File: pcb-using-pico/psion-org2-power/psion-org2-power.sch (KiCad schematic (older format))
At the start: 47 parts, among them J1 Conn_02x08_Odd_Even, J2 Conn_02x08_Odd_Even, J3 Conn_01x27_Female, J4 Conn_02x08_Odd_Even, J5 Conn_01x11_Female, J6 Conn_01x02_Female, M1 P-CHANNEL-MOSFET, M2 P-CHANNEL-MOSFET, M3 AO3401, U1 ESP32-WROOM-32, U2 AMS1117-3.3, U3 CAT24C256, U4 CAT24C256, U5 74HC595, U6 74LS245, U7 74LS245, U8 Regulator_Switching_MT3608

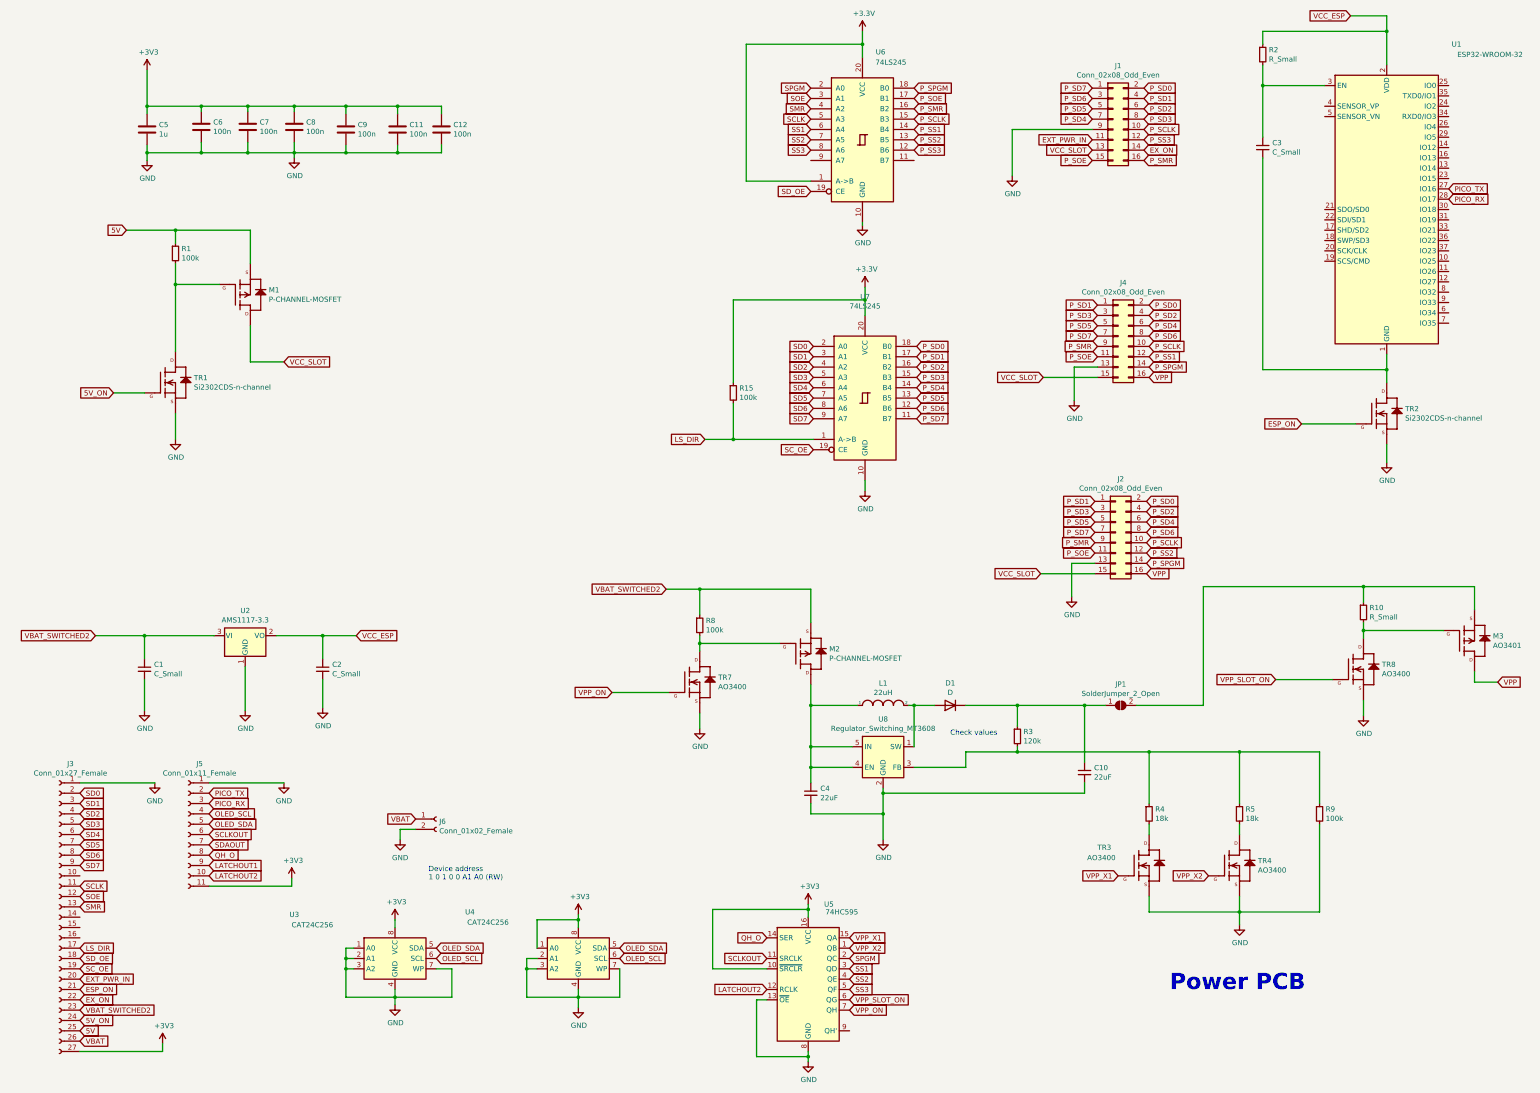
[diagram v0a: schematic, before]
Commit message: First layouts for fabrication
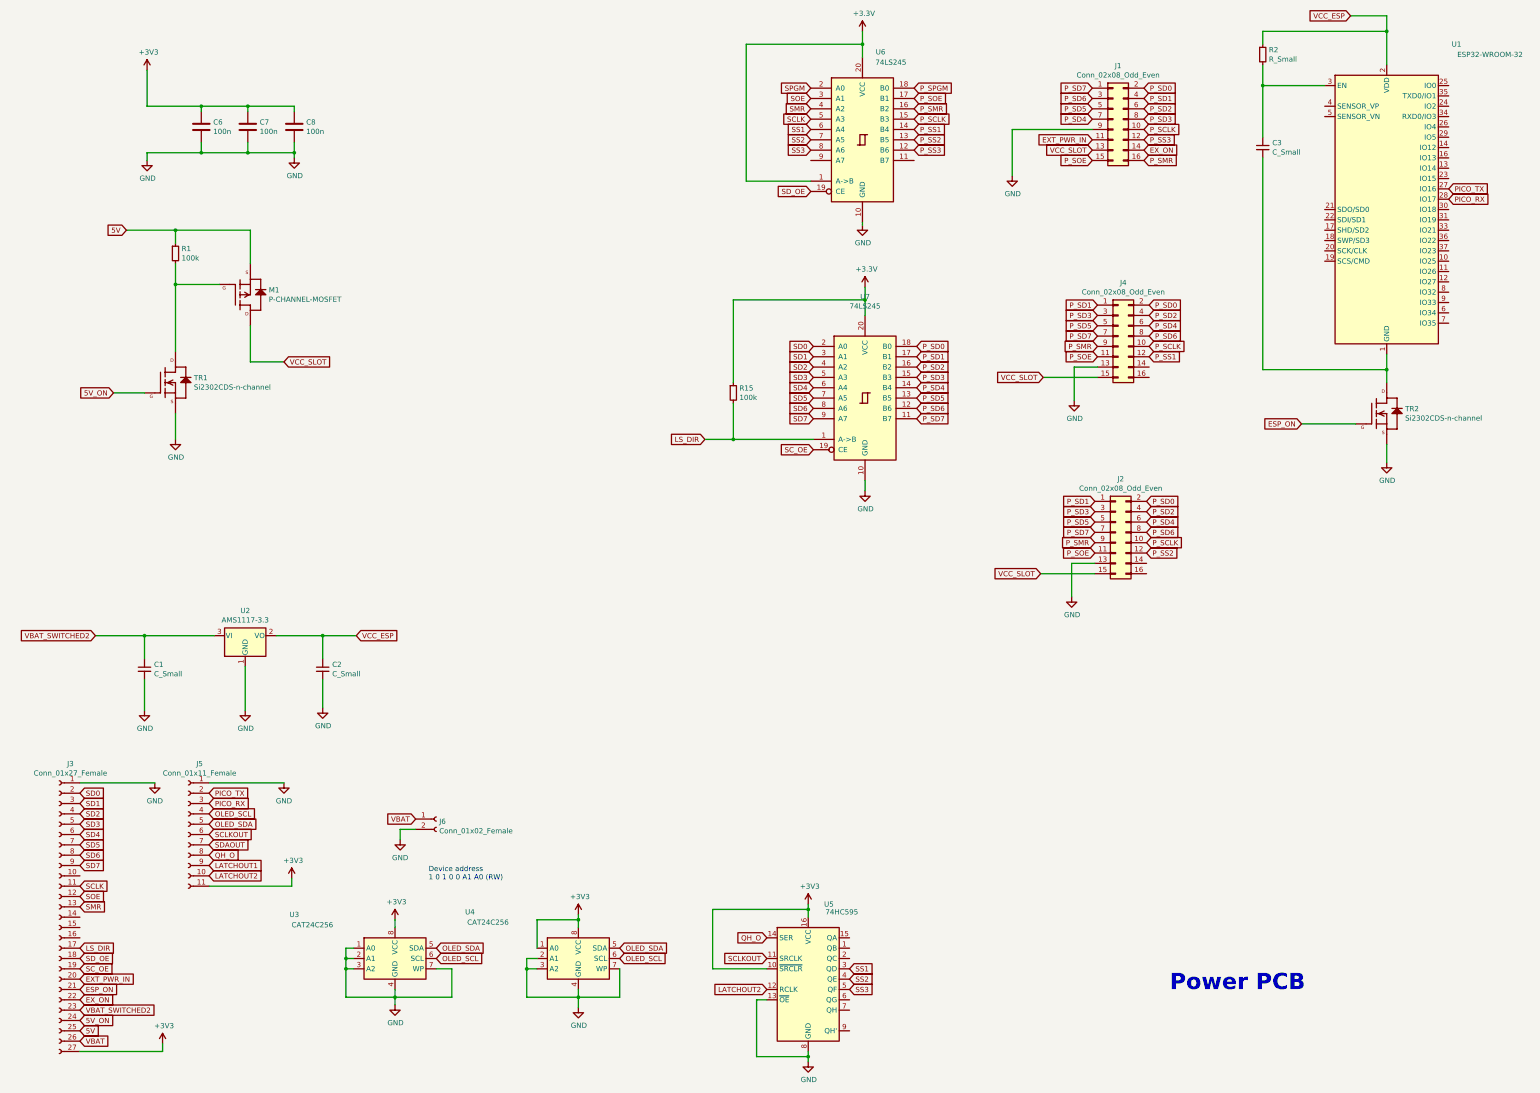
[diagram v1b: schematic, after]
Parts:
- removed C10, C4: 22uF, Capacitor_SMD:C_1210_3225Metric_Pad1.42x2.65mm_HandSolder, symbol Device:C_Small
- removed C11, C12, C9: 100n, Capacitor_SMD:C_0805_2012Metric, symbol Device:C
- removed C5: 1u, Capacitor_SMD:C_0805_2012Metric, symbol Device:C
- removed D1: D, Diode_SMD:D_SOD-123, symbol Device:D
- removed JP1: SolderJumper_2_Open, Jumper:SolderJumper-2_P1.3mm_Open_RoundedPad1.0x1.5mm, symbol Jumper:SolderJumper_2_Open
- removed L1: 22uH, Inductor_SMD:L_Coilcraft_LPS5030, symbol pspice:INDUCTOR
- removed M2: P-CHANNEL-MOSFET, Package_TO_SOT_SMD:SOT-23, symbol GeekAmmo:P-CHANNEL-MOSFET
- removed M3: AO3401, Package_TO_SOT_SMD:SOT-23, symbol GeekAmmo:P-CHANNEL-MOSFET
- removed R10: R_Small, Resistor_SMD:R_0805_2012Metric_Pad1.15x1.40mm_HandSolder, symbol Device:R_Small
- removed R3: 120k, Resistor_SMD:R_0805_2012Metric_Pad1.15x1.40mm_HandSolder, symbol Device:R_Small
- removed R4, R5: 18k, Resistor_SMD:R_0805_2012Metric_Pad1.15x1.40mm_HandSolder, symbol Device:R_Small
- removed R8, R9: 100k, Resistor_SMD:R_0805_2012Metric_Pad1.15x1.40mm_HandSolder, symbol Device:R_Small
- removed TR3, TR4, TR7, TR8: AO3400, Package_TO_SOT_SMD:SOT-23, symbol New_Library:Si2302CDS-n-channel
- removed U8: Regulator_Switching_MT3608, Package_TO_SOT_SMD:SOT-23-6, symbol cq1re1-cache:Regulator_Switching_MT3608
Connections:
- net P_SPGM: no longer J2.14 (Pin_14), J4.14 (Pin_14)
- net SPGM: no longer U5.2 (QC)
- net VPP: no longer names the net of J4.16 (Pin_16)
- net VPP: no longer J2.16 (Pin_16)
- net VPP_ON: no longer names the net of U5.7 (QH)
- net VPP_SLOT_ON: no longer names the net of U5.6 (QG)
- net VPP_X1: no longer names the net of U5.15 (QA)
- net VPP_X2: no longer names the net of U5.1 (QB)
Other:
- note removed: "Check values\n"
